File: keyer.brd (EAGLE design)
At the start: 68.2 x 30.5 mm, 52 parts, among them IC1 TINY22P, IC2 7805TV, T1 BC547, T2 BC547, T3 BC547, T4 BC547, T5 BC547, T6 BC547

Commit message: update...
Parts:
- C1, C2: value 68pF -> 22pF*
- R1, R2: value 4.7M -> 1M
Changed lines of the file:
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@@
 </autorouter>
 <elements>
-<element name="C1" library="rcl" package="C050-025X075" value="68pF" x="48.26" y="22.86" rot="R90"/>
-<element name="C2" library="rcl" package="C050-025X075" value="68pF" x="45.72" y="22.86" rot="R90"/>
+<element name="C1" library="rcl" package="C050-025X075" value="22pF*" x="48.26" y="22.86" rot="R90"/>
+<element name="C2" library="rcl" package="C050-025X075" value="22pF*" x="45.72" y="22.86" rot="R90"/>
 <element name="C3" library="rcl" package="C075-032X103" value="100nF" x="43.18" y="21.59" rot="R90"/>
 <element name="IC1" library="atmel" package="DIL08" value="TINY22P" x="39.37" y="11.43" rot="R270">
@@
 <element name="JP2" library="pinhead" package="1X02" value="paddle" x="46.99" y="15.24"/>
 <element name="JP5" library="pinhead" package="1X02" value="LED" x="34.29" y="2.54" rot="R180"/>
-<element name="R1" library="rcl" package="0204/5" value="4.7M" x="45.72" y="10.16" rot="R90"/>
-<element name="R2" library="rcl" package="0204V" value="4.7M" x="48.26" y="8.89" rot="R90"/>
+<element name="R1" library="rcl" package="0204/5" value="1M" x="45.72" y="10.16" rot="R90"/>
+<element name="R2" library="rcl" package="0204V" value="1M" x="48.26" y="8.89" rot="R90"/>
 <element name="R3" library="rcl" package="0204/5" value="10k" x="38.1" y="17.78"/>
 <element name="R4" library="rcl" package="0204/5" value="4.7k" x="22.86" y="7.62" rot="R270"/>

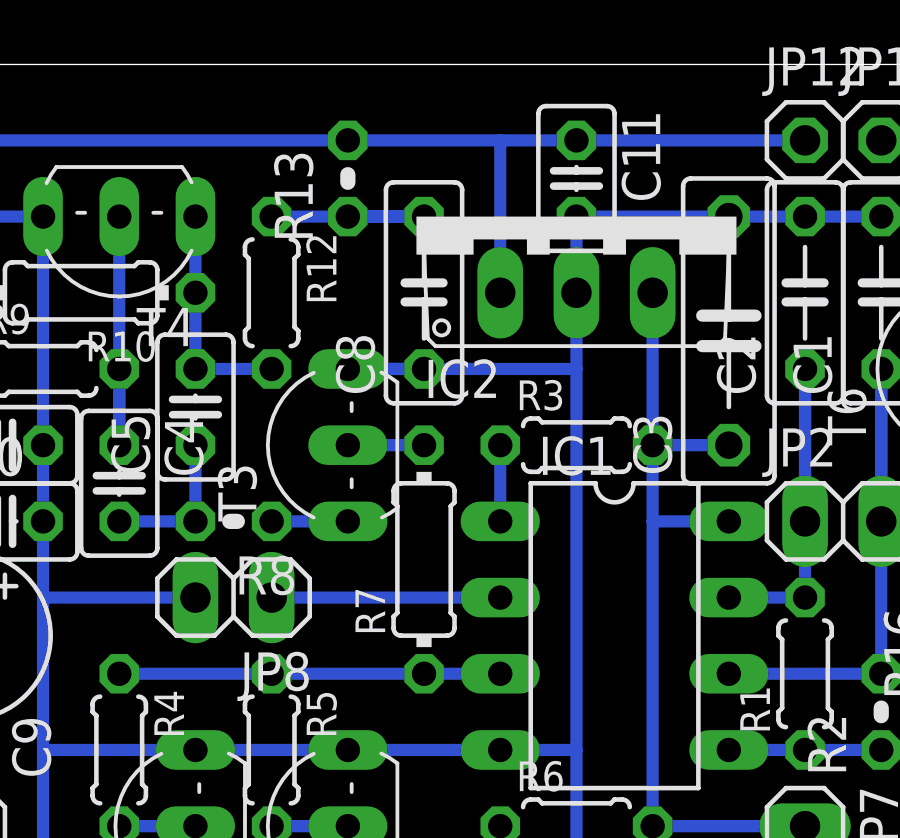
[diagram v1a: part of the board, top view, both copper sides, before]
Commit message: Cleanup.
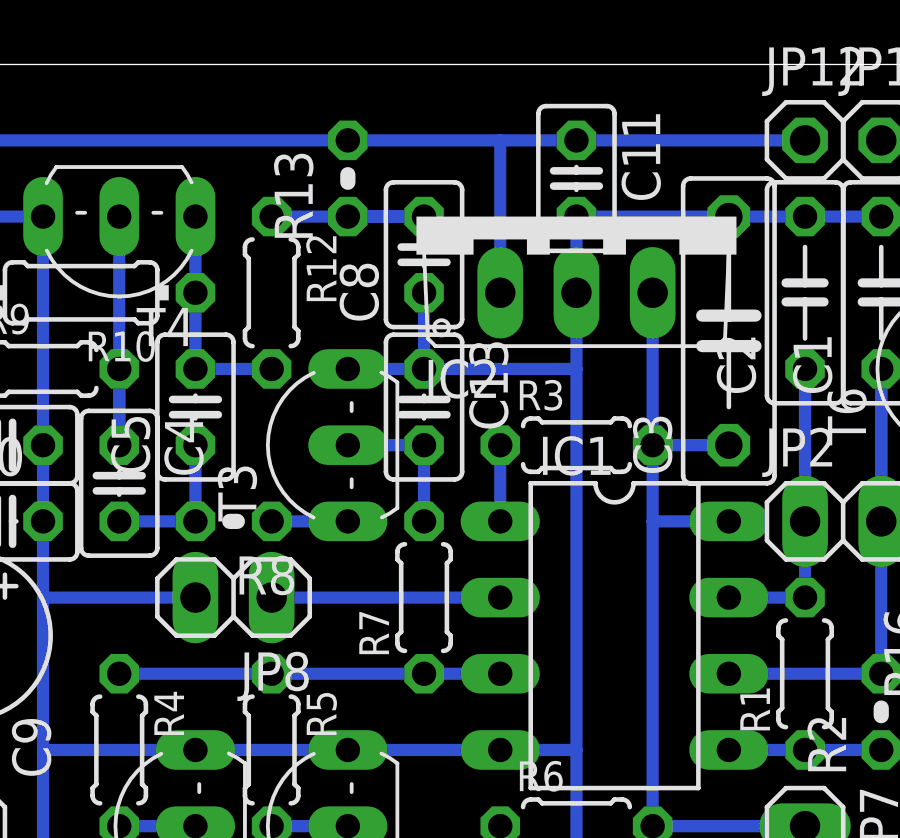
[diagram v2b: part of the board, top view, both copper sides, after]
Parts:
- added C13: 100nF*, rcl:C025-025X050
- C8: device rcl:C050-025X075 -> rcl:C025-025X050
- R7: device rcl:0204/7 -> rcl:0204/5
- moved R7 1.27 mm to (33.0, 12.7)
- moved C8 1.27 mm to (33.0, 24.1)
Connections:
- net GND: now also C13.1
- net N$14: now also C13.2
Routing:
- net N$14: track 2.54 -> 5.08 mm
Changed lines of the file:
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@@
 <element name="T2" library="transistor-neu-to92" package="TO92-CBE" value="BC547" x="30.48" y="5.08" rot="R90"/>
 <element name="T3" library="transistor-neu-to92" package="TO92-CBE" value="BC547" x="30.48" y="17.78" rot="R90"/>
-<element name="R7" library="rcl" package="0204/7" value="4.7k" x="33.02" y="13.97" rot="R90"/>
+<element name="R7" library="rcl" package="0204/5" value="4.7k" x="33.02" y="12.7" rot="R90"/>
 <element name="JP6" library="pinhead" package="1X02" value="OUT" x="11.43" y="10.16"/>
 <element name="JP7" library="pinhead" package="1X02" value="5V" x="45.72" y="3.81" rot="R270"/>
@@
 <element name="T4" library="transistor-neu-to92" package="TO92-CBE" value="BC547" x="22.86" y="25.4" rot="R180"/>
 <element name="R12" library="rcl" package="0204/5" value="3.3k" x="27.94" y="22.86" rot="R270"/>
-<element name="C8" library="rcl" package="C050-025X075" value="100nF" x="33.02" y="22.86" rot="R90"/>
+<element name="C8" library="rcl" package="C025-025X050" value="100nF" x="33.02" y="24.13" rot="R90"/>
 <element name="R13" library="rcl" package="0204V" value="10" x="30.48" y="26.67" rot="R90"/>
 <element name="C9" library="rcl" package="E2,5-6" value="10uF" x="17.78" y="11.43" rot="R270"/>
@@
 <element name="JP11" library="pinhead" package="1X01" value="SW-1" x="48.26" y="27.94"/>
 <element name="JP12" library="pinhead" package="1X01" value="SW-2" x="45.72" y="27.94"/>
+<element name="C13" library="rcl" package="C025-025X050" value="100nF*" x="33.02" y="19.05" rot="R270"/>
 </elements>
 <signals>
@@
 <wire x1="35.56" y1="7.62" x2="38.1" y2="7.62" width="0.4064" layer="16"/>
 <wire x1="38.1" y1="7.62" x2="38.1" y2="20.32" width="0.4064" layer="16"/>
+<wire x1="38.1" y1="20.32" x2="38.1" y2="22.86" width="0.4064" layer="16"/>
 <wire x1="25.4" y1="7.62" x2="30.48" y2="7.62" width="0.4064" layer="16"/>
 <wire x1="30.48" y1="7.62" x2="35.56" y2="7.62" width="0.4064" layer="16"/>
@@
 <contactref element="C11" pad="2"/>
 <contactref element="JP6" pad="2"/>
-<wire x1="30.48" y1="20.32" x2="38.1" y2="20.32" width="0.4064" layer="16"/>
-<wire x1="38.1" y1="20.32" x2="38.1" y2="22.86" width="0.4064" layer="16"/>
 <wire x1="25.4" y1="7.62" x2="20.32" y2="7.62" width="0.4064" layer="16"/>
 <wire x1="20.32" y1="7.62" x2="20.32" y2="12.7" width="0.4064" layer="16"/>
 <wire x1="38.1" y1="25.4" x2="38.1" y2="22.86" width="0.4064" layer="16"/>
-<wire x1="30.48" y1="20.32" x2="33.02" y2="20.32" width="0.4064" layer="16"/>
 <wire x1="20.32" y1="2.54" x2="20.32" y2="7.62" width="0.4064" layer="16"/>
 <contactref element="JP3" pad="1"/>
@@
 <wire x1="48.26" y1="25.4" x2="53.34" y2="25.4" width="0.4064" layer="16"/>
 <wire x1="50.8" y1="22.86" x2="53.34" y2="22.86" width="0.4064" layer="16"/>
+<contactref element="C13" pad="1"/>
+<wire x1="30.48" y1="20.32" x2="33.02" y2="20.32" width="0.4064" layer="16"/>
+<wire x1="33.02" y1="20.32" x2="38.1" y2="20.32" width="0.4064" layer="16"/>
+<wire x1="33.02" y1="20.32" x2="33.02" y2="22.86" width="0.4064" layer="16"/>
 </signal>
 <signal name="N$5">
@@
 <contactref element="T3" pad="B"/>
 <contactref element="R7" pad="2"/>
+<contactref element="C13" pad="2"/>
 <wire x1="30.48" y1="17.78" x2="33.02" y2="17.78" width="0.4064" layer="16"/>
+<wire x1="33.02" y1="17.78" x2="33.02" y2="15.24" width="0.4064" layer="16"/>
 </signal>
 <signal name="VCC">
